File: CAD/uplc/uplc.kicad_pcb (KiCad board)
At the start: 4 copper layers, 31.1 x 21 mm, 57 parts, among them J1 Conn_01x06_Pin, J2 SM12B-GHS-TB(LF)(SN), K1 G6K-2F-Y, K2 G6K-2F-Y, U1 AP63201WU, U2 ULN2803QN, U3 ESP32-C3-WROOM-02, Y1 32.568khz 3.2x1.5 12.5pf

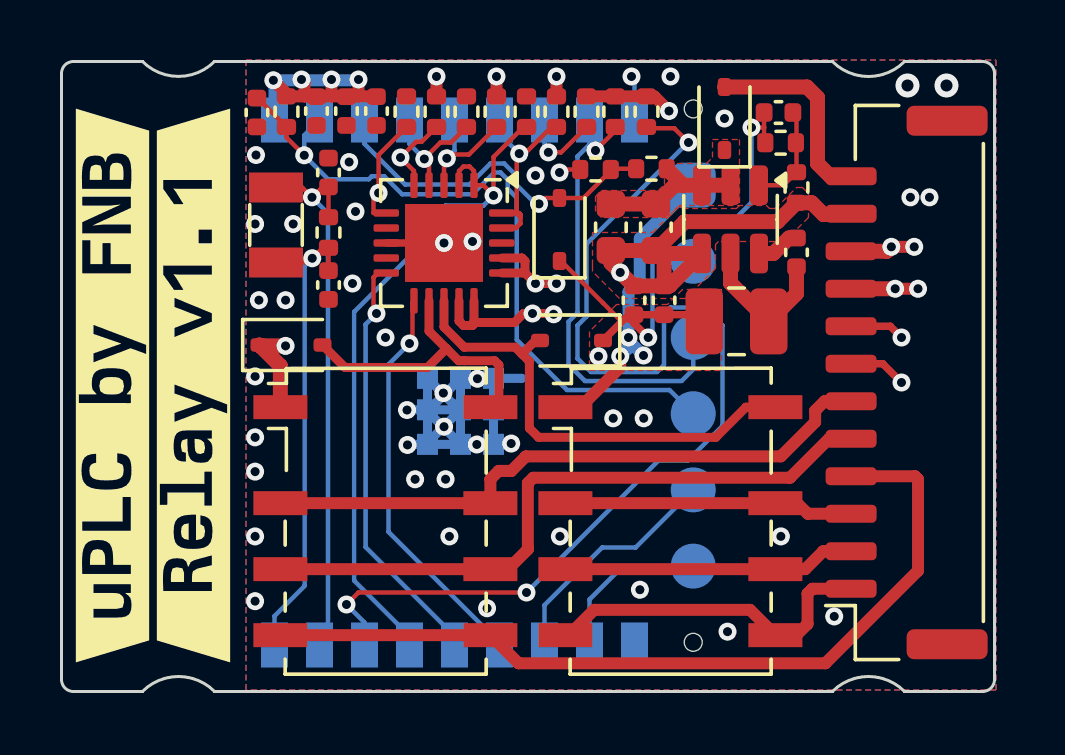
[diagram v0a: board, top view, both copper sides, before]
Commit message: Rev 1.2
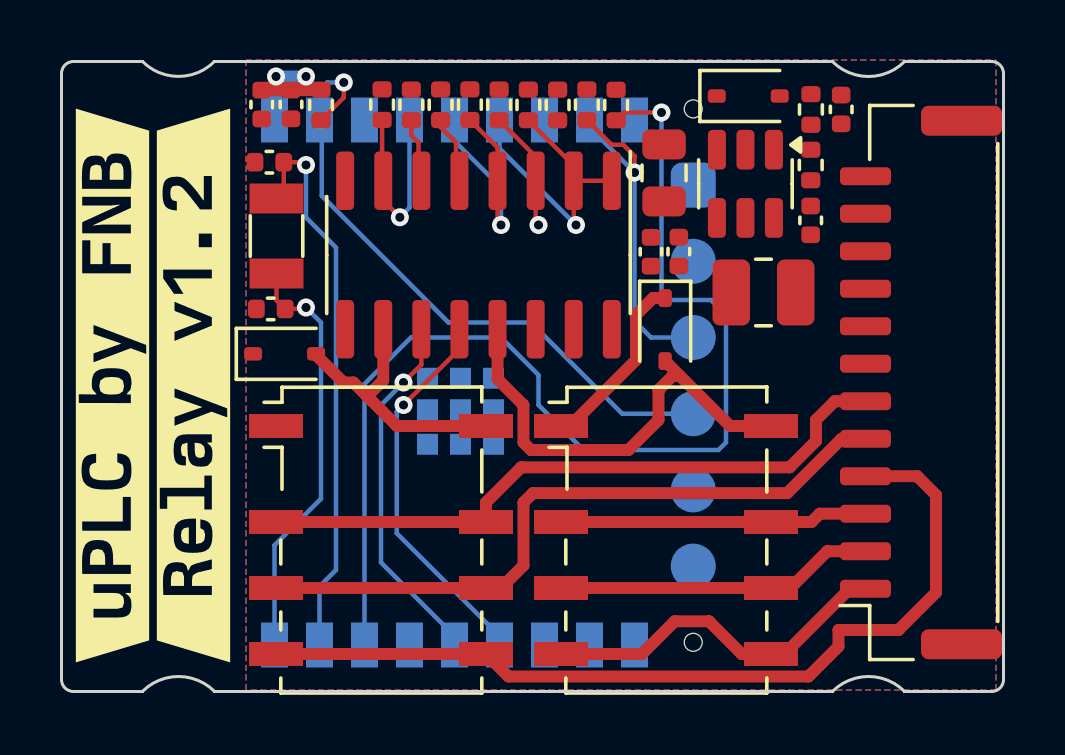
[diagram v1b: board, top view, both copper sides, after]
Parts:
- removed C10, C6: 0.1uF, Capacitor_SMD:C_0402_1005Metric
- removed C7: 4.7uF, Capacitor_SMD:C_0603_1608Metric
- removed D3: 1N5819WS, Diode_SMD:D_SOD-323
- removed R13: 1M, Resistor_SMD:R_0402_1005Metric
- removed R3: 13.7k, Resistor_SMD:R_0402_1005Metric
- removed R6: 316k, Resistor_SMD:R_0402_1005Metric
- removed kibuzzard-65D60D86: G***, kibuzzard-65D60D86
- added kibuzzard-65D6FF37: G***, kibuzzard-65D6FF37, F.Cu at (104.5, 82.6)
- C5: value 4.7uF -> 10uF; footprint Capacitor_SMD:C_0603_1608Metric -> Capacitor_SMD:C_0805_2012Metric
- U2: value ULN2803QN -> TBD62003AFWG; footprint Package_DFN_QFN:QFN-20-1EP_4x4mm_P0.5mm_EP2.6x2.6mm -> Package_SO:SOIC-16_3.9x9.9mm_P1.27mm
- moved C3 3.83 mm to (106.8, 73.2)
- moved D2 3.14 mm to (120.2, 80.7), turned to -90 degrees
- moved R10 2.82 mm to (110.8, 73.2)
- moved C9 2.09 mm to (126.1, 73.4), turned to -90 degrees
- moved C1 2.08 mm to (107.1, 80.0), turned to 0 degrees
- moved C4 2.00 mm to (107.0, 75.2), turned to 180 degrees
- moved C5 1.83 mm to (120.2, 75.5)
- moved C8 1.71 mm to (119.8, 78.1)
- moved C12 1.70 mm to (120.7, 78.1)
- moved R14 1.50 mm to (125.1, 73.4), turned to 90 degrees
- moved L1 1.32 mm to (123.5, 79.5)
- moved U1 1.28 mm to (122.9, 75.9)
- moved U2 1.22 mm to (114.0, 78.2)
- moved R1 1.17 mm to (108.8, 73.2)
- moved C2 1.17 mm to (125.1, 77.1)
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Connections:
- U2 pad 1: LI3 -> LI12
- U2 pad 10: LO7 -> RO1
- U2 pad 11: LO6 -> LO7
- U2 pad 12: RO1 -> LO6
- U2 pad 15: HO2 -> HO1
- U2 pad 2: LI3 -> LI12
- U2 pad 3: LI4 -> LI3
- U2 pad 4: LI5 -> LI4
- U2 pad 7: (no net) -> LI5
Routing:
- net +3.3V: track 78.8 -> 11.5 mm, vias 12 -> 2
- net GND: track 42.0 -> 0.00 mm, vias 47 -> 0
- net HI2: track 27.2 -> 2.16 mm, vias 2 -> 0
- net HI1: track 26.0 -> 2.28 mm, vias 2 -> 0
- net LI3: track 23.3 -> 4.04 mm
- net HO2: track 18.8 -> 0.00 mm, vias 4 -> 0
- net HO1: track 17.0 -> 0.00 mm, vias 4 -> 0
- net ADC: track 11.9 -> 0.00 mm, vias 1 -> 0
- net TX: track 7.88 -> 0.00 mm
- net +VDC: track 6.74 -> 0.00 mm
- net RX: track 5.44 -> 0.00 mm
- net /VIN_P: track 5.02 -> 0.00 mm
- net /SW: track 4.99 -> 0.00 mm
- net LI4: track 4.41 -> 8.07 mm
- net /FB: track 3.47 -> 0.00 mm
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- removed copper zone on F.Cu, net +3.3V
- removed copper zone on F.Cu, net /VIN_P
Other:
- board size 31.1 x 21 mm -> 31.4 x 21 mm
